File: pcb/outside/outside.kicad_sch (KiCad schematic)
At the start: 27 parts, among them J1 USB_C_Receptacle_USB2.0_16P, J2 RJ12, U3 USBLC6-2SC6, U4 AMS1117-3.3

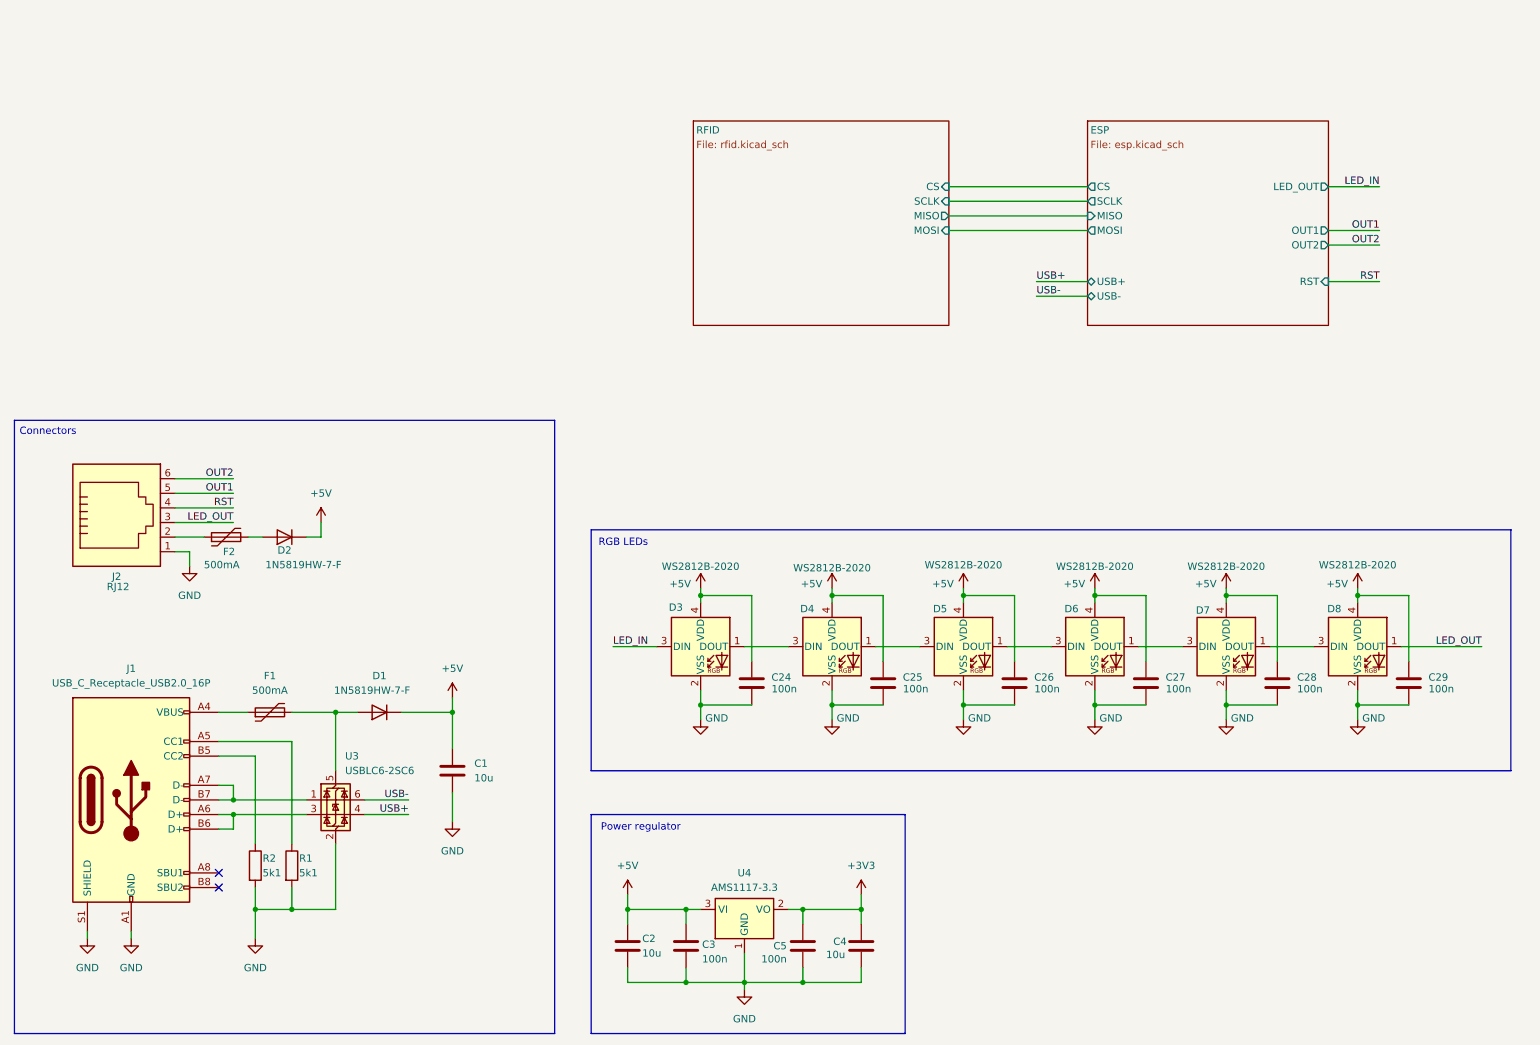
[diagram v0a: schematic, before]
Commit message: feat: add testpoints and rearrange schematic
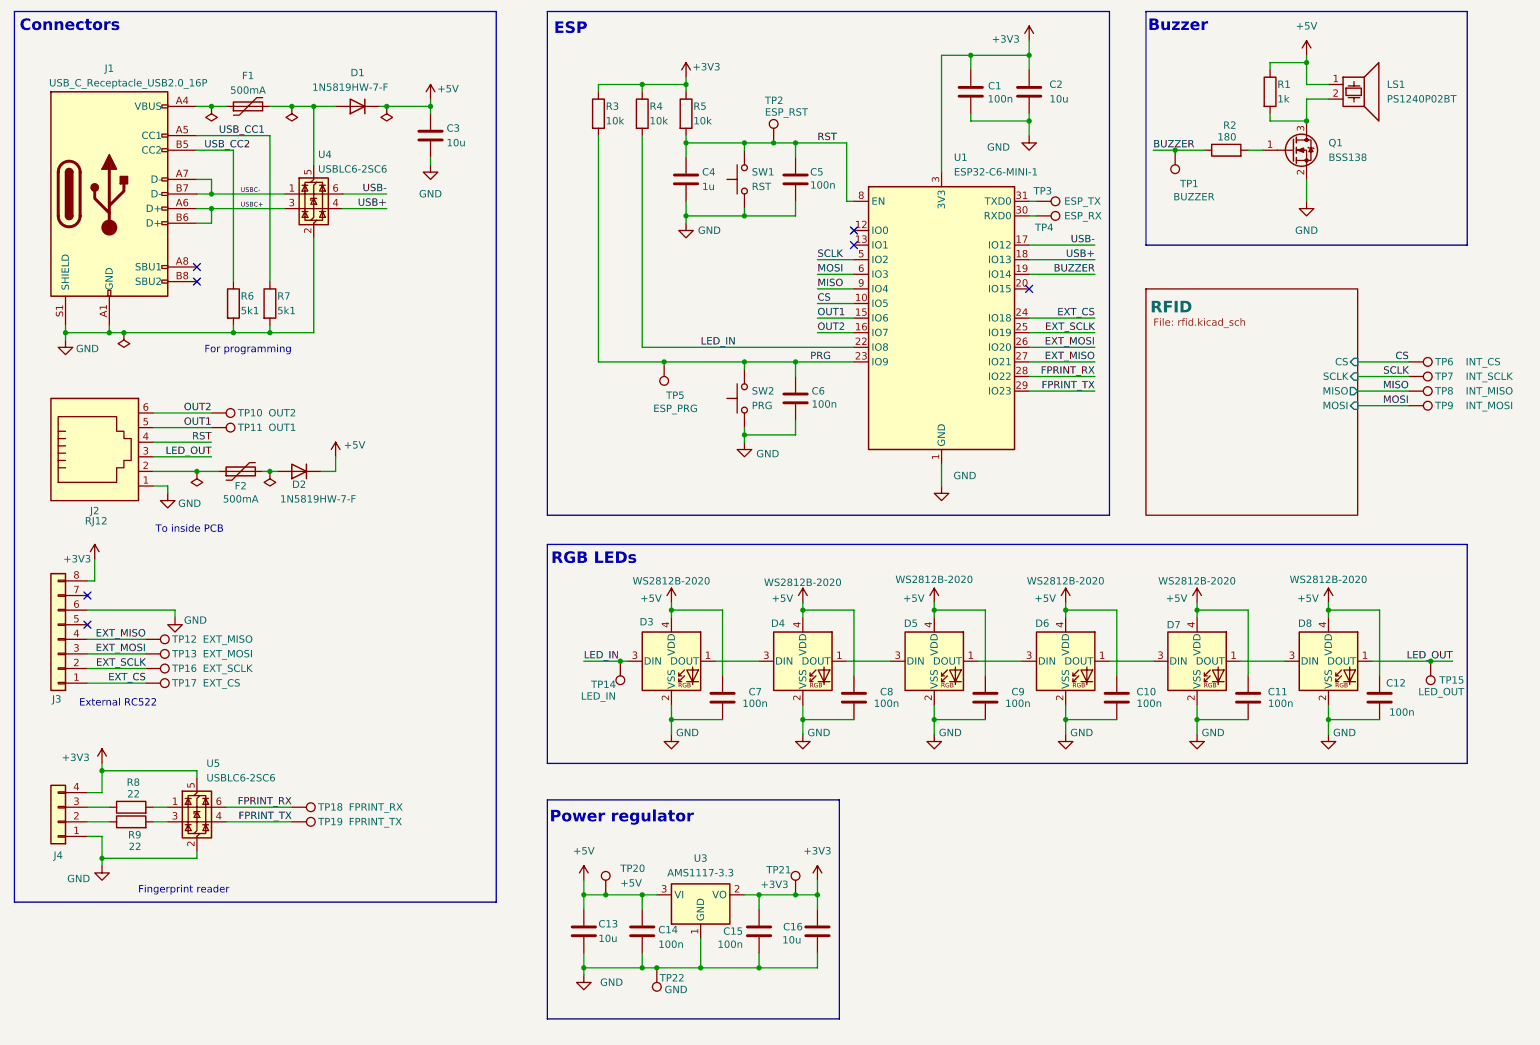
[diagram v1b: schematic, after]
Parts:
- removed U3: USBLC6-2SC6, Package_TO_SOT_SMD:SOT-23-6, symbol Power_Protection:USBLC6-2SC6
- added C2, C3: 10u, Capacitor_SMD:C_0603_1608Metric, symbol Device:C
- added C4: 1u, Capacitor_SMD:C_0603_1608Metric, symbol Device:C
- added C5, C6: 100n, Capacitor_SMD:C_0603_1608Metric, symbol Device:C
- added J3: Conn_01x08, Connector_PinSocket_2.54mm:PinSocket_1x08_P2.54mm_Vertical, symbol Connector_Generic:Conn_01x08
- added J4: Conn_01x04, Connector_JST:JST_XH_B4B-XH-A_1x04_P2.50mm_Vertical, symbol Connector_Generic:Conn_01x04
- added LS1: PS1240P02BT, belepteto:PS1240P02BT, symbol Device:Speaker_Crystal
- added Q1: BSS138, Package_TO_SOT_SMD:SOT-23, symbol Transistor_FET:BSS138
- added R3, R4, R5: 10k, Resistor_SMD:R_0603_1608Metric, symbol Device:R
- added R6, R7: 5k1, Resistor_SMD:R_0603_1608Metric, symbol Device:R
- added R8, R9: 22, Resistor_SMD:R_0603_1608Metric, symbol Device:R
- added SW1: RST, Button_Switch_SMD:SW_SPST_TL3342, symbol Switch:SW_Push
- added SW2: PRG, Button_Switch_SMD:SW_SPST_TL3342, symbol Switch:SW_Push
- added TP1: BUZZER, TestPoint:TestPoint_Pad_D1.0mm, symbol Connector:TestPoint
- added TP10: OUT2, TestPoint:TestPoint_Pad_D1.0mm, symbol Connector:TestPoint
- added TP11: OUT1, TestPoint:TestPoint_Pad_D1.0mm, symbol Connector:TestPoint
- added TP12: EXT_MISO, TestPoint:TestPoint_Pad_D1.0mm, symbol Connector:TestPoint
- added TP13: EXT_MOSI, TestPoint:TestPoint_Pad_D1.0mm, symbol Connector:TestPoint
- added TP14: LED_IN, TestPoint:TestPoint_Pad_D1.0mm, symbol Connector:TestPoint
- added TP15: LED_OUT, TestPoint:TestPoint_Pad_D1.0mm, symbol Connector:TestPoint
- added TP16: EXT_SCLK, TestPoint:TestPoint_Pad_D1.0mm, symbol Connector:TestPoint
- added TP17: EXT_CS, TestPoint:TestPoint_Pad_D1.0mm, symbol Connector:TestPoint
- added TP18: FPRINT_RX, TestPoint:TestPoint_Pad_D1.0mm, symbol Connector:TestPoint
- added TP19: FPRINT_TX, TestPoint:TestPoint_Pad_D1.0mm, symbol Connector:TestPoint
- added TP2: ESP_RST, TestPoint:TestPoint_Pad_D1.0mm, symbol Connector:TestPoint
- added TP20: +5V, TestPoint:TestPoint_Pad_D1.0mm, symbol Connector:TestPoint
- added TP21: +3V3, TestPoint:TestPoint_Pad_D1.0mm, symbol Connector:TestPoint
- added TP22: GND, TestPoint:TestPoint_Pad_D1.0mm, symbol Connector:TestPoint
- added TP3: ESP_TX, TestPoint:TestPoint_Pad_D1.0mm, symbol Connector:TestPoint
- added TP4: ESP_RX, TestPoint:TestPoint_Pad_D1.0mm, symbol Connector:TestPoint
- added TP5: ESP_PRG, TestPoint:TestPoint_Pad_D1.0mm, symbol Connector:TestPoint
- added TP6: INT_CS, TestPoint:TestPoint_Pad_D1.0mm, symbol Connector:TestPoint
- added TP7: INT_SCLK, TestPoint:TestPoint_Pad_D1.0mm, symbol Connector:TestPoint
- added TP8: INT_MISO, TestPoint:TestPoint_Pad_D1.0mm, symbol Connector:TestPoint
- added TP9: INT_MOSI, TestPoint:TestPoint_Pad_D1.0mm, symbol Connector:TestPoint
- added U1: ESP32-C6-MINI-1, RF_Module:ESP32-C6-MINI-1, symbol RF_Module:ESP32-C6-MINI-1
- added U4, U5: USBLC6-2SC6, Package_TO_SOT_SMD:SOT-23-6, symbol Power_Protection:USBLC6-2SC6
- C1: value 10u -> 100n
- R1: value 5k1 -> 1k
- R2: value 5k1 -> 180
- renumbered C27 to C10, C28 to C11, C29 to C12, C2 to C13, C3 to C14, C5 to C15, C4 to C16, C24 to C7, C25 to C8, C26 to C9, U4 to U3
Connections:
- net +3V3: now also C1.1, C2.1, J3.8 (Pin_8), J4.4 (Pin_4), R3.1, R4.1, R5.1, TP21.1, U1.3 (3V3), U5.5 (VBUS)
- net +5V: now also R1.1, C3.1, LS1.1, TP20.1; no longer C1.1
- net GND: now also C2.2, C3.2, C4.2, C5.1, C6.1, J3.6 (Pin_6), J4.1 (Pin_1), Q1.2 (S), R6.2, R7.2, SW1.1, SW2.1, TP22.1, U1.1 (GND), U1.11 (GND), U1.14 (GND), U1.2 (GND), U1.36 (GND), U1.37 (GND), U1.38 (GND), U1.39 (GND), U1.40 (GND), U1.41 (GND), U1.42 (GND), U1.43 (GND), U1.44 (GND), U1.45 (GND), U1.46 (GND), U1.47 (GND), U1.48 (GND), U1.49 (GND), U1.50 (GND), U1.51 (GND), U1.52 (GND), U1.53 (GND), U4.2 (GND), U5.2 (GND); no longer R1.2, R2.2
- net LED_IN: now also R4.2, TP14.1, U1.22 (IO8)
- net LED_OUT: now also TP15.1
- net OUT1: now also TP11.1, U1.15 (IO6)
- net OUT2: now also TP10.1, U1.16 (IO7)
- net RST: now also C4.1, C5.2, R5.2, SW1.2, TP2.1, U1.8 (EN)
- net USB+: now also U1.18 (IO13), U4.4 (I/O2)
- net USB-: now also U1.17 (IO12), U4.6 (I/O1)
- net USB_CC1: now reaches J1.A5 (CC1)
- net USB_CC1: now also R7.1; no longer R1.1
- net BUZZER: now reaches R2.1
- net BUZZER: now also TP1.1, U1.19 (IO14); no longer J1.B5 (CC2)
- net USBC+: now reaches J1.A6 (D+), J1.B6 (D+)
- net USBC+: now also U4.3 (I/O2)
- net USBC-: now reaches J1.A7 (D-), J1.B7 (D-)
- net USBC-: now also U4.1 (I/O1)
- net at D1.2 (A), F1.2: now also U4.5 (VBUS)
- new net: R8.2, U5.1 (I/O1)
- new net: R9.2, U5.3 (I/O2)
- new net: TP3.1, U1.31 (TXD0)
- new net: J4.2 (Pin_2), R9.1
- new net: J4.3 (Pin_3), R8.1
- new net: TP4.1, U1.30 (RXD0)
- new net: Q1.1 (G), R2.2
- new net: LS1.2, Q1.3 (D), R1.2
- new net CS: TP6.1, U1.10 (IO5)
- new net EXT_CS: J3.1 (Pin_1), TP17.1, U1.24 (IO18)
- new net EXT_MISO: J3.4 (Pin_4), TP12.1, U1.27 (IO21)
- new net EXT_MOSI: J3.3 (Pin_3), TP13.1, U1.26 (IO20)
- new net EXT_SCLK: J3.2 (Pin_2), TP16.1, U1.25 (IO19)
- new net FPRINT_RX: TP18.1, U1.28 (IO22), U5.6 (I/O1)
- new net FPRINT_TX: TP19.1, U1.29 (IO23), U5.4 (I/O2)
- new net MISO: TP8.1, U1.9 (IO4)
- new net MOSI: TP9.1, U1.6 (IO3)
- new net PRG: C6.2, R3.2, SW2.2, TP5.1, U1.23 (IO9)
- new net SCLK: TP7.1, U1.5 (IO2)
- new net USB_CC2: J1.B5 (CC2), R6.1
- no-connect marks 2 -> 7
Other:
- removed sheet ESP
- note added: "Buzzer"
- note added: "ESP"
- note added: "External RC522"
- note added: "Fingerprint reader"
- note added: "For programming"
- note added: "To inside PCB"
- moved on the sheet: C10, C11, C12, C13, C14, C15, C16, C7, C8, C9, D3, D4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
